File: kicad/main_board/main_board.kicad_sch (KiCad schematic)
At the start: 8 parts

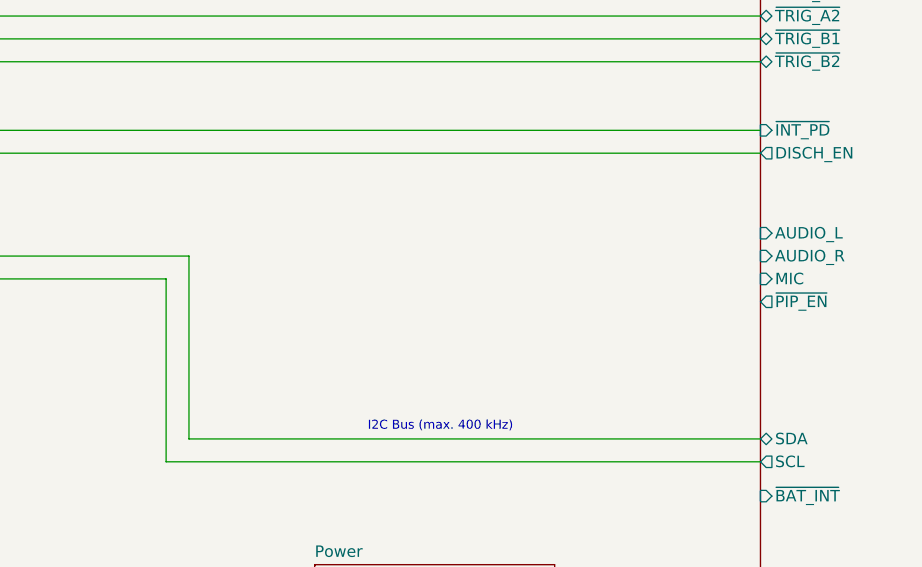
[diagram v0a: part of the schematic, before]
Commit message: add audio
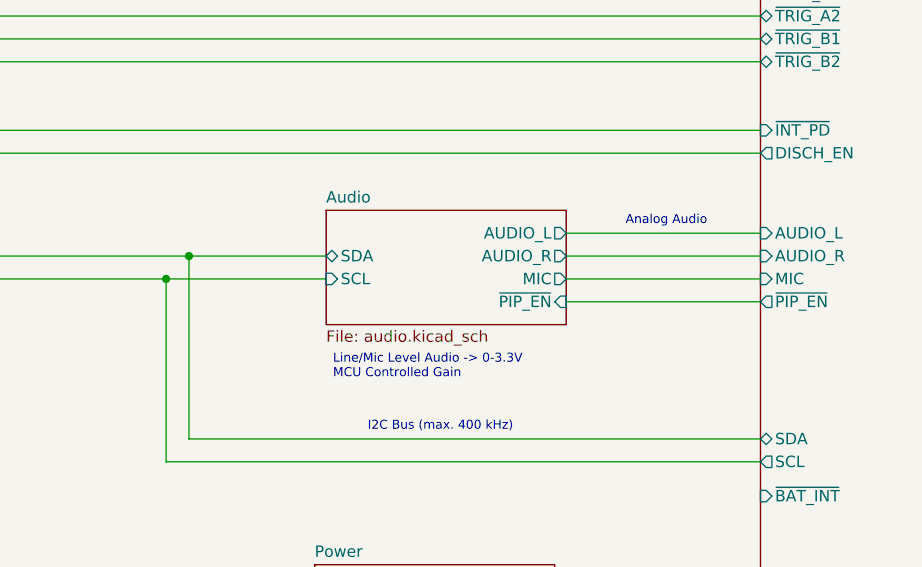
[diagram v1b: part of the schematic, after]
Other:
- added sheet Audio (audio.kicad_sch)
- note added: "Analog Audio"
- note added: "Line/Mic Level Audio -> 0-3.3V MCU Controlled Gain"
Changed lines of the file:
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@@
 		(company "saawsm")
 	)
+	(junction
+		(at 106.68 87.63)
+		(diameter 0)
+		(color 0 0 0 0)
+	)
+	(junction
+		(at 109.22 85.09)
+		(diameter 0)
+		(color 0 0 0 0)
+	)
 	(wire
 		(pts
@@
 	(wire
 		(pts
+			(xy 106.68 87.63) (xy 124.46 87.63)
+		)
+		(stroke
+			(width 0)
+			(type default)
+		)
+	)
+	(wire
+		(pts
+			(xy 151.13 90.17) (xy 172.72 90.17)
+		)
+		(stroke
+			(width 0)
+			(type default)
+		)
+	)
+	(wire
+		(pts
 			(xy 207.01 59.69) (xy 217.17 59.69)
 		)
@@
 	(wire
 		(pts
+			(xy 151.13 82.55) (xy 172.72 82.55)
+		)
+		(stroke
+			(width 0)
+			(type default)
+		)
+	)
+	(wire
+		(pts
+			(xy 151.13 87.63) (xy 172.72 87.63)
+		)
+		(stroke
+			(width 0)
+			(type default)
+		)
+	)
+	(wire
+		(pts
 			(xy 149.86 123.19) (xy 172.72 123.19)
 		)
@@
 	(wire
 		(pts
+			(xy 109.22 85.09) (xy 124.46 85.09)
+		)
+		(stroke
+			(width 0)
+			(type default)
+		)
+	)
+	(wire
+		(pts
 			(xy 68.58 87.63) (xy 106.68 87.63)
+		)
+		(stroke
+			(width 0)
+			(type default)
+		)
+	)
+	(wire
+		(pts
+			(xy 151.13 85.09) (xy 172.72 85.09)
 		)
 		(stroke
@@
 			)
 			(justify top)
+		)
+	)
+	(text "Line/Mic Level Audio -> 0-3.3V \nMCU Controlled Gain"
+		(exclude_from_sim no)
+		(at 125.222 98.806 0)
+		(effects
+			(font
+				(size 1 1)
+			)
+			(justify left bottom)
+		)
+	)
+	(text "Analog Audio"
+		(exclude_from_sim no)
+		(at 157.734 81.788 0)
+		(effects
+			(font
+				(size 1 1)
+			)
+			(justify left bottom)
 		)
 	)
@@
 				)
 			)
+		)
+	)
+	(sheet
+		(at 124.46 80.01)
+		(size 26.67 12.7)
+		(fields_autoplaced yes)
+		(stroke
+			(width 0.1524)
+			(type solid)
+		)
+		(fill
+			(color 0 0 0 0.0000)
+		)
+		(property "Sheetname" "Audio"
+			(at 124.46 79.2984 0)
+			(effects
+				(font
+					(size 1.27 1.27)
+				)
+				(justify left bottom)
+			)
+		)
+		(property "Sheetfile" "audio.kicad_sch"
+			(at 124.46 93.2946 0)
+			(effects
+				(font
+					(size 1.27 1.27)
+				)
+				(justify left top)
+			)
+		)
+		(pin "SCL" input
+			(at 124.46 87.63 180)
+			(effects
+				(font
+					(size 1.27 1.27)
+				)
+				(justify left)
+			)
+		)
+		(pin "SDA" bidirectional
+			(at 124.46 85.09 180)
+			(effects
+				(font
+					(size 1.27 1.27)
+				)
+				(justify left)
+			)
+		)
+		(pin "~{PIP_EN}" input
+			(at 151.13 90.17 0)
+			(effects
+				(font
+					(size 1.27 1.27)
+				)
+				(justify right)
+			)
+		)
+		(pin "MIC" output
+			(at 151.13 87.63 0)
+			(effects
+				(font
+					(size 1.27 1.27)
+				)
+				(justify right)
+			)
+		)
+		(pin "AUDIO_L" output
+			(at 151.13 82.55 0)
+			(effects
+				(font
+					(size 1.27 1.27)
+				)
+				(justify right)
+			)
+		)
+		(pin "AUDIO_R" output
+			(at 151.13 85.09 0)
+			(effects
+				(font
+					(size 1.27 1.27)
+				)
+				(justify right)
+			)
+		)
+		(instances
+			(project "main_board"
+				(path "/8e1f1504-76c2-49e6-9261-3c1190503f8c"
+					(page "6")
+				)
+			)

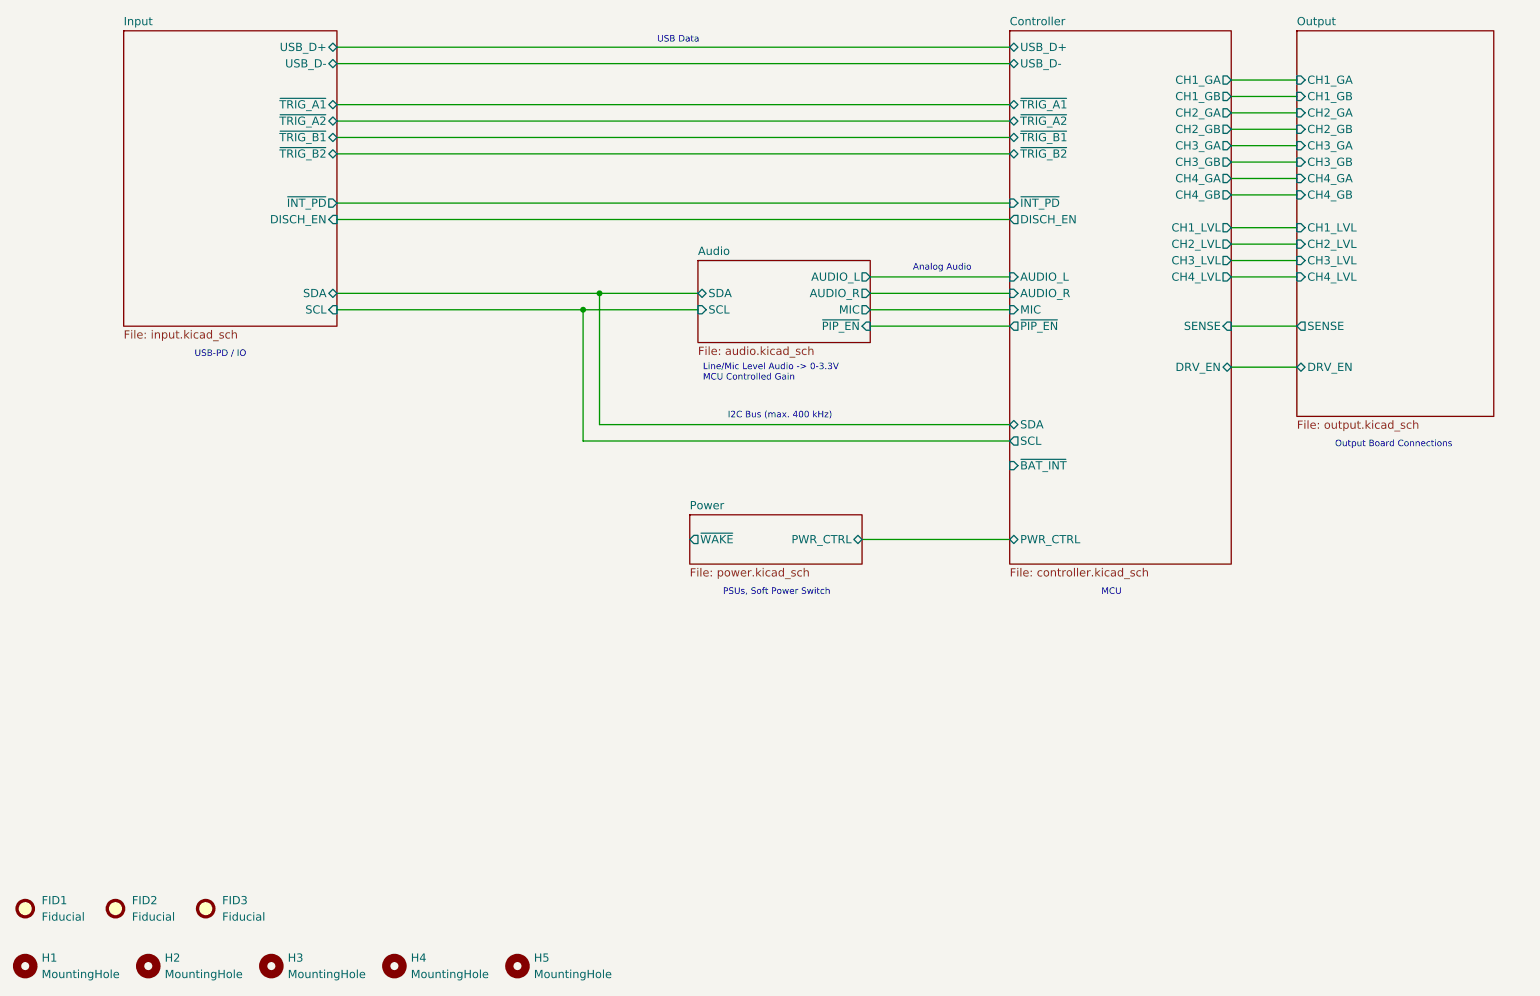
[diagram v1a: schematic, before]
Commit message: add charger
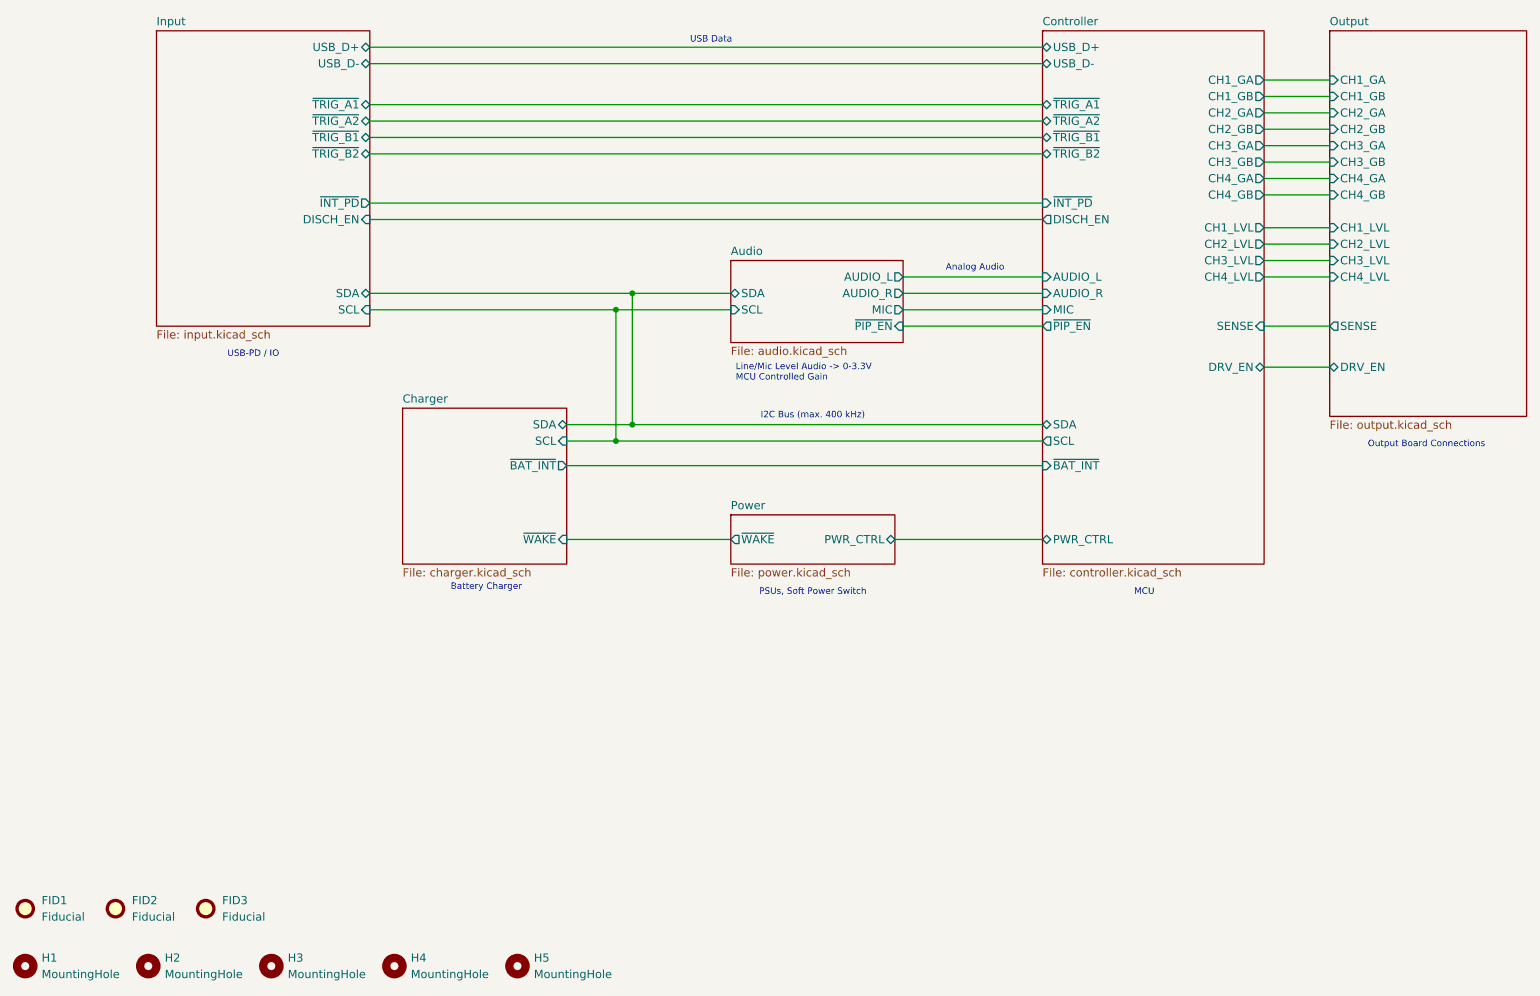
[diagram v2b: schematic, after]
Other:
- added sheet Charger (charger.kicad_sch)
- note added: "Battery Charger"
